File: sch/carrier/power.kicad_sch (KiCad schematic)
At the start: 20 parts, among them J1 1054500101, Q1 BC557, Q2 BC557

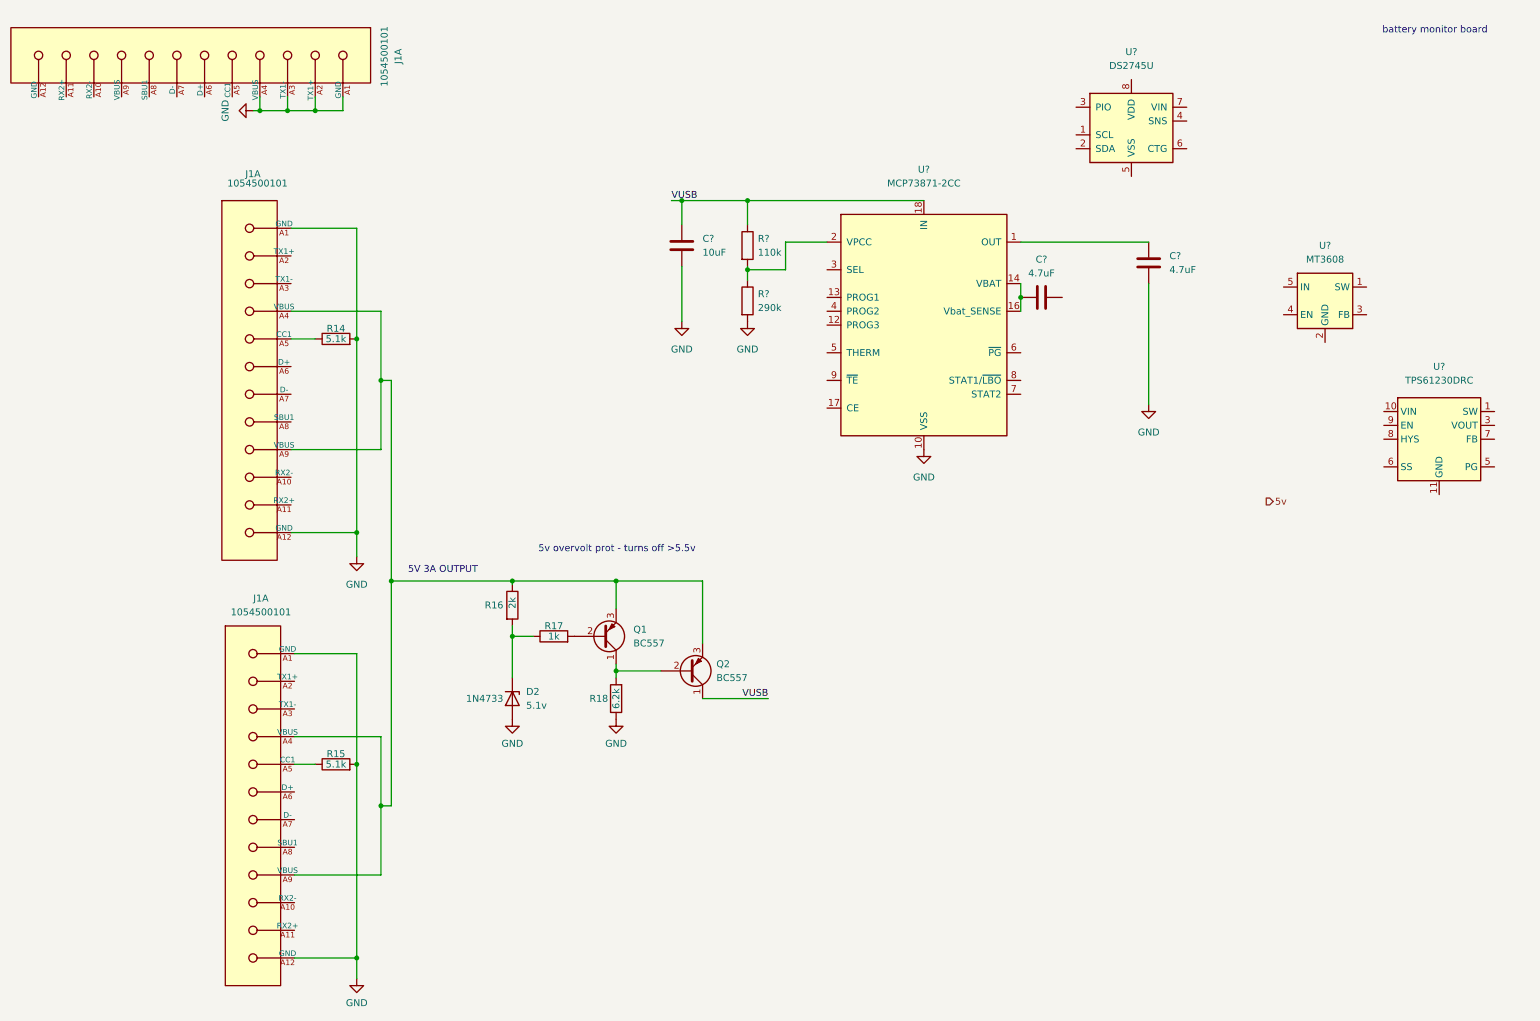
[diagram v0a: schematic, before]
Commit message: h
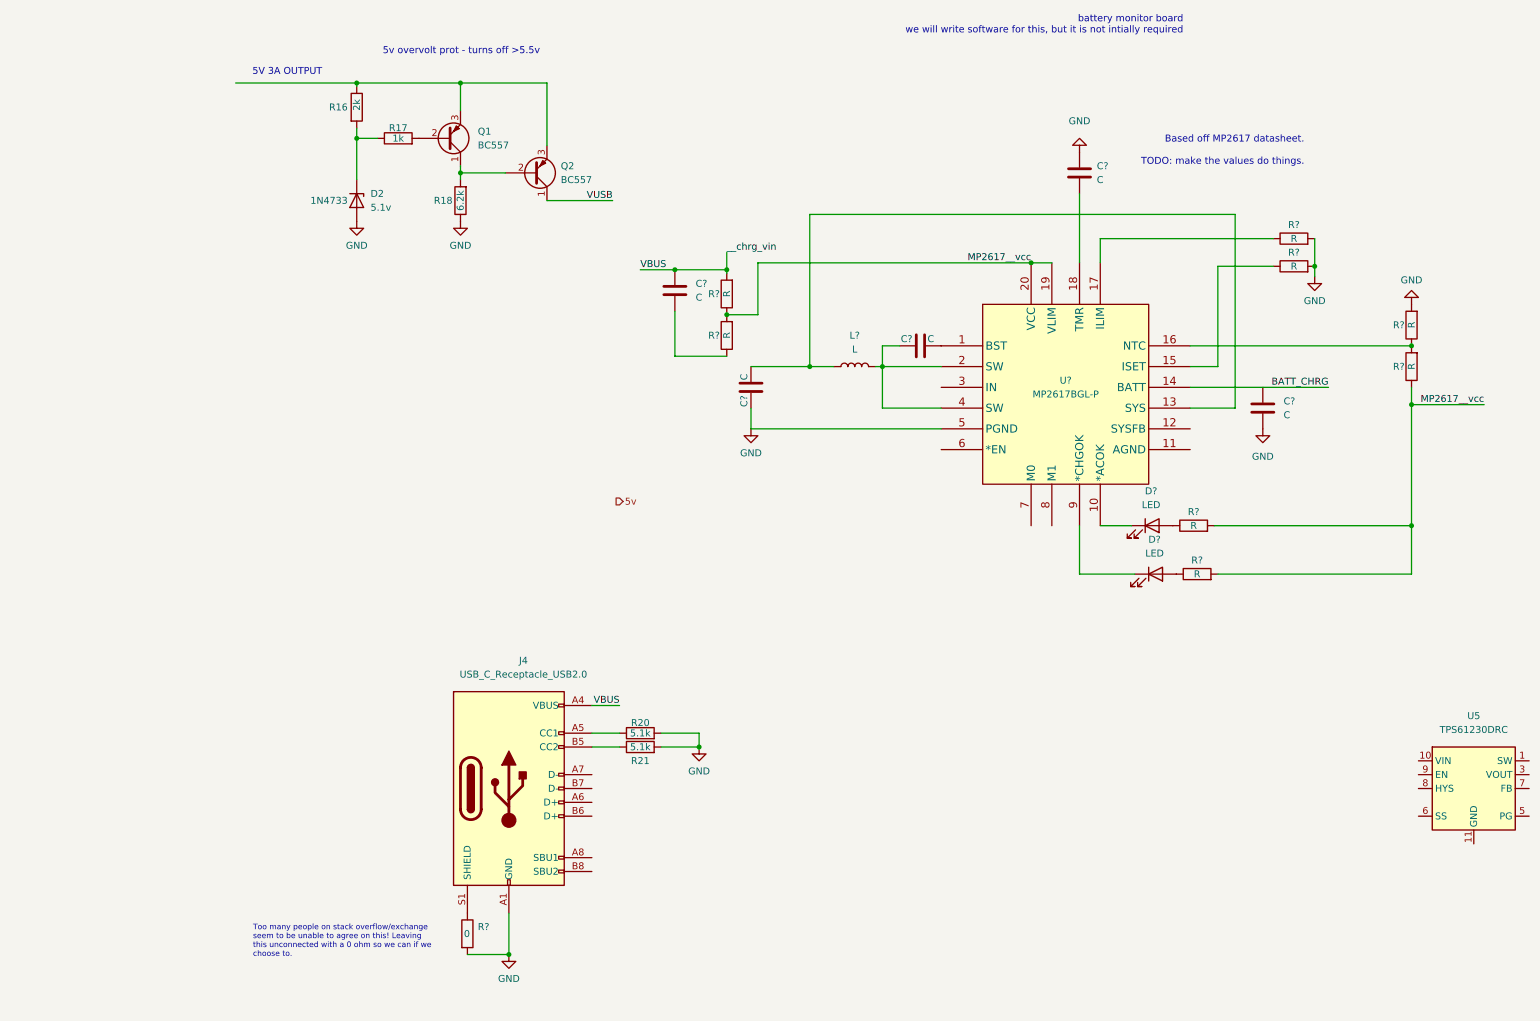
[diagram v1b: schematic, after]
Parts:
- removed C? (x2): 4.7uF, symbol Device:C
- removed C?: 10uF, symbol Device:C
- removed J1 (x3): 1054500101, MOLEXC:Molex-1054500101-MFG, symbol MOLEXC:1054500101
- removed R14, R15: 5.1k, Resistor_SMD:R_0805_2012Metric_Pad1.20x1.40mm_HandSolder, symbol Device:R
- removed R?: 110k, symbol Device:R
- removed R?: 290k, symbol Device:R
- removed U?: DS2745U, Package_SO:TSSOP-8_3x3mm_P0.65mm, symbol Battery_Management:DS2745U
- removed U?: MCP73871-2CC, Package_DFN_QFN:QFN-20-1EP_4x4mm_P0.5mm_EP2.5x2.5mm, symbol Battery_Management:MCP73871-2CC
- removed U?: MT3608, Package_TO_SOT_SMD:SOT-23-6, symbol Regulator_Switching:MT3608
- added C? (x5): C, symbol Device:C
- added D? (x2): LED, symbol Device:LED
- added J4: USB_C_Receptacle_USB2.0, Connector_USB:USB_C_Receptacle_JAE_DX07S016JA1R1500, symbol Connector:USB_C_Receptacle_USB2.0
- added L?: L, symbol Device:L
- added R20, R21: 5.1k, Resistor_SMD:R_0805_2012Metric_Pad1.20x1.40mm_HandSolder, symbol Device:R
- added R? (x8): R, symbol Device:R
- added R?: 0, symbol Device:R
- added U?: MP2617BGL-P, symbol MP:MP2617BGL-P
- gave numbers to parts that had none: 1
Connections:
- net GND: now also C?.1, C?.1, C?.2, J4.A1 (GND), J4.A12 (GND), J4.B1 (GND), J4.B12 (GND), R20.2, R21.2, R?.2, R?.2, R?.2, R?.2, U?.5 (PGND)
- new net: C?.2, L?.1, U?.13 (SYS)
- new net: J4.A5 (CC1), R20.1
- new net: D?.1 (K), U?.10 (*ACOK)
- new net: D?.2 (A), R?.1 (x2)
- new net: J4.B5 (CC2), R21.1
- new net: J4.S1 (SHIELD), R?.1
- new net: C?.2, R?.1
- new net: R?.1, U?.17 (ILIM)
- new net: R?.1, R?.2, U?.16 (NTC)
- new net: D?.1 (K), U?.9 (*CHGOK)
- new net: R?.1, U?.15 (ISET)
- new net: C?.1, L?.2, U?.2 (SW), U?.4 (SW)
- new net: C?.2, U?.1 (BST)
- new net: C?.2, U?.18 (TMR)
- new net BATT_CHRG: U?.14 (BATT)
- new net MP2617__vcc: R?.1, R?.1, R?.2, R?.2, R?.2, U?.19 (VLIM), U?.20 (VCC)
- new net VBUS: C?.1, J4.A4 (VBUS), J4.A9 (VBUS), J4.B4 (VBUS), J4.B9 (VBUS), R?.2
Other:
- note added: "Based off MP2617 datasheet. TODO: make the values do things."
- note added: "Too many people on stack overflow/exchange seem to be unable to agree on this! Leaving this unconnected with a 0 ohm so we can if we choose to."
- note added: "battery monitor board we will write software for this, but it is not intially required"
- note removed: "battery monitor board"
- moved on the sheet: D2, Q1, Q2, R16, R17, R18, U5
